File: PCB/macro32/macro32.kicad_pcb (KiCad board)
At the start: 2 copper layers, 103.9 x 100 mm, 58 parts, among them J1 OLED, J2 OLED, J3 Magnetic connector, J4 Magnetic connector, J5 Magnetic connector, J6 Magnetic connector, SW1 RST, U1 SuperMini_NRF52840

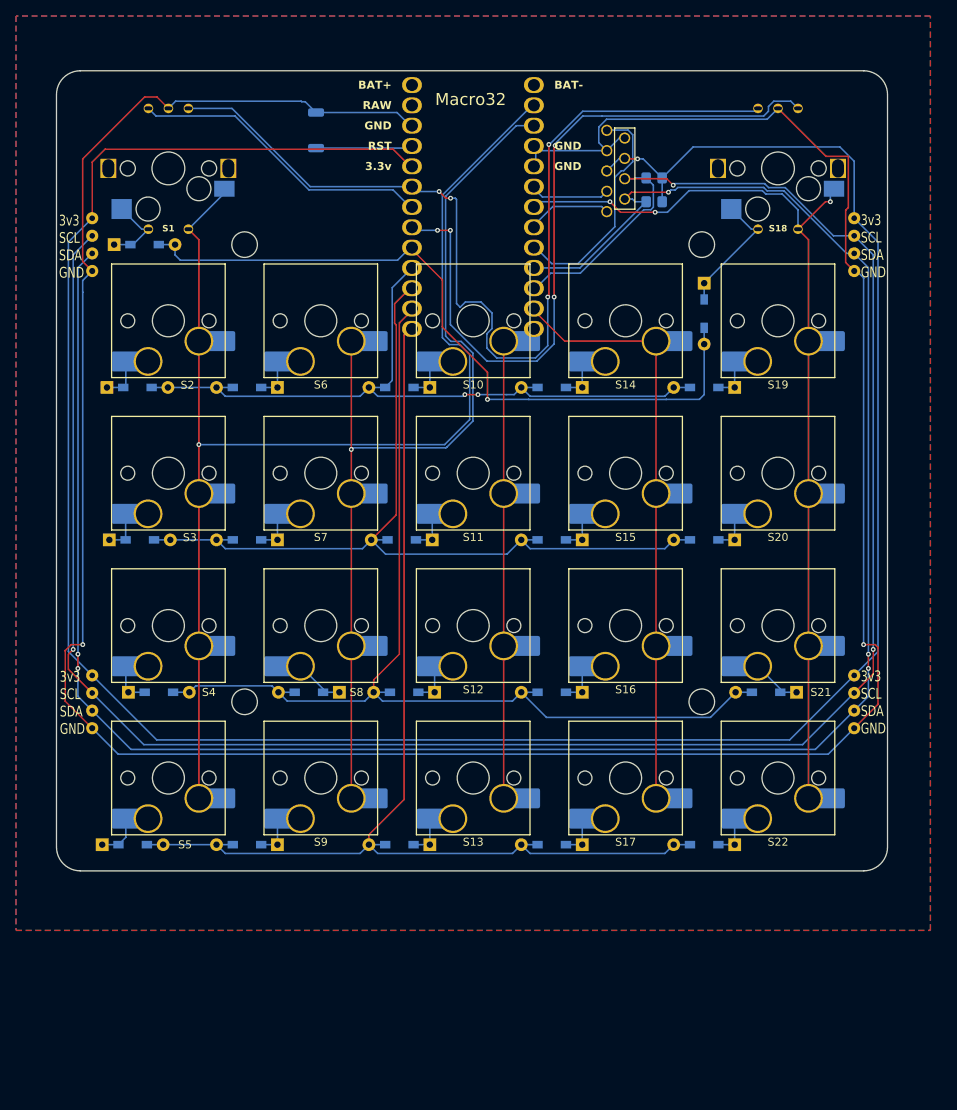
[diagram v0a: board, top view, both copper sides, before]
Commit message: macro32_v2_schem&pcb
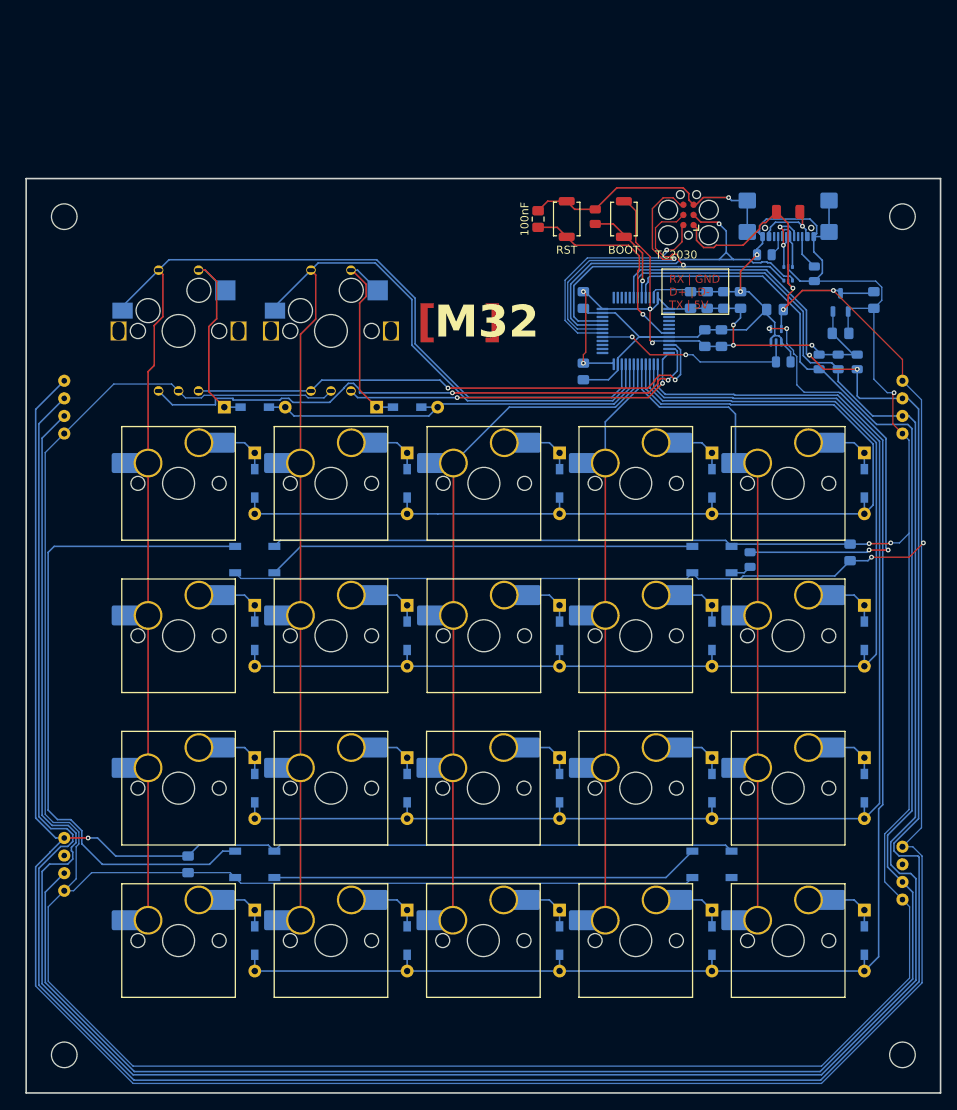
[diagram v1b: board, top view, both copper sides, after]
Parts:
- removed R1, R2: 10k, Resistor_SMD:R_0805_2012Metric_Pad1.20x1.40mm_HandSolder
- removed S1: Rotary_Encoder_Switch, KillrOfLife_Keyboard:keyswitch_cherrymx_hotswap_1u_rotary_encoder_ec12
- added C1: 1μF, Capacitor_SMD:C_0805_2012Metric_Pad1.18x1.45mm_HandSolder, B.Cu at (150.0, 65.8)
- added C10: 100nF, Capacitor_SMD:C_0805_2012Metric_Pad1.18x1.45mm_HandSolder, B.Cu at (131.0, 70.5)
- added C11: 100nF, Capacitor_SMD:C_0805_2012Metric_Pad1.18x1.45mm_HandSolder, B.Cu at (133.4, 65.8)
- added C12: 100nF, Capacitor_SMD:C_0805_2012Metric_Pad1.18x1.45mm_HandSolder, B.Cu at (137.7, 66.9)
- added C13: 100nF, Capacitor_SMD:C_0805_2012Metric_Pad1.18x1.45mm_HandSolder, B.Cu at (147.0, 97.3)
- added C14: 100nF, Capacitor_SMD:C_0805_2012Metric_Pad1.18x1.45mm_HandSolder, B.Cu at (64.3, 136.3)
- added C2: 1μF, Capacitor_SMD:C_0805_2012Metric_Pad1.18x1.45mm_HandSolder, B.Cu at (128.9, 70.5)
- added C3: 4,7μF, Capacitor_SMD:C_0805_2012Metric_Pad1.18x1.45mm_HandSolder, B.Cu at (127.1, 65.8)
- added C4: 1μF, Capacitor_SMD:C_0805_2012Metric_Pad1.18x1.45mm_HandSolder, B.Cu at (145.9, 69.9)
- added C5: 100nF, Capacitor_SMD:C_0805_2012Metric_Pad1.18x1.45mm_HandSolder, B.Cu at (113.7, 74.7)
- added C6: 100nF, Capacitor_SMD:C_0805_2012Metric_Pad1.18x1.45mm_HandSolder, F.Cu at (108.1, 55.6)
- added C7: 100nF, Capacitor_SMD:C_0805_2012Metric_Pad1.18x1.45mm_HandSolder, B.Cu at (131.3, 65.8)
- added C8: 100nF, Capacitor_SMD:C_0805_2012Metric_Pad1.18x1.45mm_HandSolder, B.Cu at (113.7, 65.8)
- added C9: 100nF, Capacitor_SMD:C_0805_2012Metric_Pad1.18x1.45mm_HandSolder, B.Cu at (129.2, 65.8)
- added D23: LED_WS2812B, KillrOfLife_Components:LED_WS2812B, B.Cu at (129.8, 98.2)
- added D24: LED_WS2812B, KillrOfLife_Components:LED_WS2812B, B.Cu at (72.6, 98.2)
- added D25: LED_WS2812B, KillrOfLife_Components:LED_WS2812B, B.Cu at (72.6, 136.3)
- added D26: LED_WS2812B, KillrOfLife_Components:LED_WS2812B, B.Cu at (129.8, 136.3)
- added F1: 500mA, KillrOfLife_Components:Resistor_1206, F.Cu at (139.3, 54.7)
- added R10: 10kΩ, KillrOfLife_Components:Resistor_0805, B.Cu at (143.2, 73.5)
- added R11: 100kΩ, KillrOfLife_Components:Resistor_0805, B.Cu at (138.7, 73.5)
- added R12: 470Ω, KillrOfLife_Components:Resistor_0805, B.Cu at (134.5, 98.2)
- added R5: 5k1Ω, KillrOfLife_Components:Resistor_0805, B.Cu at (136.3, 60.1)
- added R6: 5k1Ω, KillrOfLife_Components:Resistor_0805, B.Cu at (142.6, 62.5)
- added R7: 10kΩ, KillrOfLife_Components:Resistor_0805, F.Cu at (115.2, 55.3)
- added R8: 2.2kΩ, KillrOfLife_Components:Resistor_0805, B.Cu at (147.9, 73.5)
- added R9: 2.2kΩ, KillrOfLife_Components:Resistor_0805, B.Cu at (145.6, 73.5)
- added S23: Rotary_Encoder_Switch, KillrOfLife_Keyboard:keyswitch_cherrymx_hotswap_1u_rotary_encoder_ec12_1, B.Cu at (82.2, 69.6)
- added SW2: BOOT, Button_Switch_SMD:SW_SPST_TS-1088-xR020, F.Cu at (118.8, 55.6)
- added U2: STM32F07, Package_QFP:LQFP-48_7x7mm_P0.5mm, B.Cu at (120.3, 69.6)
- added U3: LDO, Package_TO_SOT_SMD:SOT-23-3, B.Cu at (145.9, 66.0)
- added U4: 74AHC1G125, Package_TO_SOT_SMD:SOT-353_SC-70-5, B.Cu at (137.8, 70.2)
- D1, D10, D11, D12, D13, D14, D15, D16, D17, D18, D19, D2, D20, D21, D22, D3, D4, D5, D6, D7, D8, D9: footprint KillrOfLife_Components:SMD_SOD123_Leaded -> KillrOfLife_Components:Diode_combo
- H1, H2, H3, H4: moved to B.Cu
- J1: value OLED -> USB_C_Receptacle_USB2.0_16P; footprint KillrOfLife_Connectors:OLED_4Pin -> Connector_USB:USB_C_Receptacle_GCT_USB4110; moved to B.Cu
- J2: value OLED -> TC2030; footprint KillrOfLife_Connectors:OLED_5Pin -> Connector:Tag-Connect_TC2030-IDC-FP_2x03_P1.27mm_Vertical
- J3, J5: footprint Library:fakemag4pin90degFemale -> KillrOfLife_Connectors:fakemag4pin90degFemale
- J4, J6: footprint Library:fakemag4pin90degMale -> KillrOfLife_Connectors:fakemag4pin90degFemale
- S10, S11, S12, S13, S14, S15, S16, S17, S19, S2, S20, S21, S22, S3, S4, S5, S7, S8, S9: footprint ScottoKeebs_Hotswap:Hotswap_MX_Plated_1.00u -> KillrOfLife_Keyboard:Hotswap_MX_Plated_1.00u
- S18: value Rotary_Encoder_Switch -> Keyswitch; footprint KillrOfLife_Keyboard:keyswitch_cherrymx_hotswap_1u_rotary_encoder_ec12 -> KillrOfLife_Keyboard:Hotswap_MX_Plated_1.00u; moved to F.Cu
- S6: value Keyswitch -> Rotary_Encoder_Switch; footprint ScottoKeebs_Hotswap:Hotswap_MX_Plated_1.00u -> KillrOfLife_Keyboard:keyswitch_cherrymx_hotswap_1u_rotary_encoder_ec12_1; moved to B.Cu
- SW1: moved to F.Cu
- U1: value SuperMini_NRF52840 -> USBLC6; footprint KillrOfLife_MCU:SuperMini_NRF52850_pro_micro -> Package_TO_SOT_SMD:SOT-666
- moved J4 125.5 mm to (48.8, 136.3)
- moved J5 107.8 mm to (153.6, 79.1), turned to 180 degrees
- moved S18 98.1 mm to (120.3, 145.8)
- moved S10 79.5 mm to (82.2, 145.8), turned to 0 degrees
- moved S14 79.5 mm to (101.2, 145.8), turned to 0 degrees
- moved D22 66.1 mm to (91.7, 79.1), turned to 180 degrees
- moved D5 56.8 mm to (72.6, 79.1)
- moved H4 50.8 mm to (153.6, 160.1), turned to 180 degrees
- moved H3 49.6 mm to (48.8, 160.1), turned to 180 degrees
- moved U1 40.0 mm to (139.3, 62.5), turned to -90 degrees
- moved J1 38.5 mm to (139.3, 54.1), turned to 0 degrees
- moved D20 36.9 mm to (148.8, 126.8), turned to 90 degrees
- moved D19 36.9 mm to (148.8, 107.7), turned to 90 degrees
- moved D2 34.3 mm to (72.6, 107.7), turned to 90 degrees
- moved D3 34.2 mm to (72.6, 126.8), turned to 90 degrees
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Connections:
- D1 pad 1: ROW0 -> ROW1
- D18 pad 1: ROW0 -> ROW1
- D19 pad 1: ROW1 -> ROW2
- D2 pad 1: ROW1 -> ROW2
- D20 pad 1: ROW2 -> ROW3
- D21 pad 1: ROW3 -> ROW4
- D22 pad 1: ROW4 -> ROW0
- D3 pad 1: ROW2 -> ROW3
- D4 pad 1: ROW3 -> ROW4
- D5 pad 1: ROW4 -> ROW0
- J2 pad 1: MOSI -> +5V
- J2 pad 2: SCK -> TX
- J2 pad 3: +3V3 -> D-
- J2 pad 4: GND -> D+
- J2 pad 5: CS -> GND
- J3 pad 1: +3V3 -> +5V
- J4 pad 1: GND -> +5V
- J4 pad 2: SDA -> unconnected-(J4-P2-Pad2)
- J4 pad 3: SCL -> INT
- J4 pad 4: +3V3 -> GND
- J5 pad 1: +3V3 -> GND
- J5 pad 2: SCL -> SDA
- J5 pad 3: SDA -> SCL
- J5 pad 4: GND -> +5V
- J6 pad 2: SDA -> INT
- J6 pad 3: SCL -> unconnected-(J6-P3-Pad3)
- J6 pad 4: +3V3 -> +5V
- S10 pad 1: COL2 -> COL1
- S10 pad 2: Net-(D10-A) -> Net-(D9-A)
- S11 pad 2: Net-(D11-A) -> Net-(D10-A)
- S12 pad 2: Net-(D12-A) -> Net-(D11-A)
- S13 pad 2: Net-(D13-A) -> Net-(D12-A)
- S14 pad 1: COL3 -> COL2
- S14 pad 2: Net-(D14-A) -> Net-(D13-A)
- S15 pad 2: Net-(D15-A) -> Net-(D14-A)
- S16 pad 2: Net-(D16-A) -> Net-(D15-A)
- S17 pad 2: Net-(D17-A) -> Net-(D16-A)
- S19 pad 2: Net-(D19-A) -> Net-(D18-A)
- S2 pad 2: Net-(D2-A) -> Net-(D1-A)
- S20 pad 2: Net-(D20-A) -> Net-(D19-A)
- S21 pad 2: Net-(D21-A) -> Net-(D20-A)
- S22 pad 2: Net-(D22-A) -> Net-(D21-A)
- S3 pad 2: Net-(D3-A) -> Net-(D2-A)
- S4 pad 2: Net-(D4-A) -> Net-(D3-A)
- S5 pad 2: Net-(D5-A) -> Net-(D4-A)
- S7 pad 2: Net-(D7-A) -> Net-(D6-A)
- S8 pad 2: Net-(D8-A) -> Net-(D7-A)
- S9 pad 2: Net-(D9-A) -> Net-(D8-A)
- U1 pad 1: unconnected-(U1-BAT--Pad1) -> USB D+
- U1 pad 2: COL0 -> GND
- U1 pad 3: COL1 -> USB D-
- U1 pad 4: GND -> D-
- U1 pad 5: GND -> +5V
- U1 pad 6: SCK -> D+
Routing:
- net +5V: track 0.00 -> 514.4 mm, vias 0 -> 6
- net GND: track 348.4 -> 633.2 mm, vias 2 -> 6
- net INT: track 0.00 -> 250.9 mm
- net +3V3: track 314.8 -> 93.4 mm, vias 1 -> 7
- net Net-(D24-DOUT): track 0.00 -> 83.7 mm
- net encoders: track 123.4 -> 67.3 mm, vias 4 -> 2
- net Net-(R12-Pad1): track 0.00 -> 55.5 mm, vias 0 -> 4
- net Net-(D23-DOUT): track 0.00 -> 53.6 mm
- net Net-(D25-DOUT): track 0.00 -> 53.6 mm
- net SCL: track 276.8 -> 326.9 mm, vias 3 -> 2
- net SDA: track 269.7 -> 319.5 mm, vias 5 -> 0
- net D-: track 0.00 -> 49.0 mm, vias 0 -> 1
- net D+: track 0.00 -> 48.0 mm, vias 0 -> 1
- net encoder2_1: track 90.7 -> 44.2 mm, vias 4 -> 2
- net ROW4: track 143.3 -> 187.4 mm
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- removed copper zone on B.Cu, net GND
- removed copper zone on F.Cu, net GND
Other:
- board size 103.9 x 100 mm -> 114.3 x 114.3 mm
- board text added: "Hello"
- board text added: "M32"
- board text added: "RX | GND D+ | D- TX | 5V"
- board text added: "[ ]"
- board text removed: "3v3 SCL SDA GND"
- board text removed: "Macro32"
